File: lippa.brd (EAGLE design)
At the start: 50 x 80 mm, 149 parts, among them K1 629105136821, X1 B4B-PH-K-S, X10 PIIKKIRIMA-3, X11 B8B-PH-K-S, X2 B4B-PH-K-S, X3 B4B-PH-K-S, X4 B4B-PH-K-S, X5 LIITTIMET_X3815-10, X7 PIIKKIRIMA-3, X8 B6B-PH-K-S, X9 PIIKKIRIMA-3, Y1 EKE_PTH3.2-6.5SQ, Y2 EKE_PTH3.2-6.5SQ, Y3 EKE_PTH3.2-6.5SQ, Y4 EKE_PTH3.2-6.5SQ

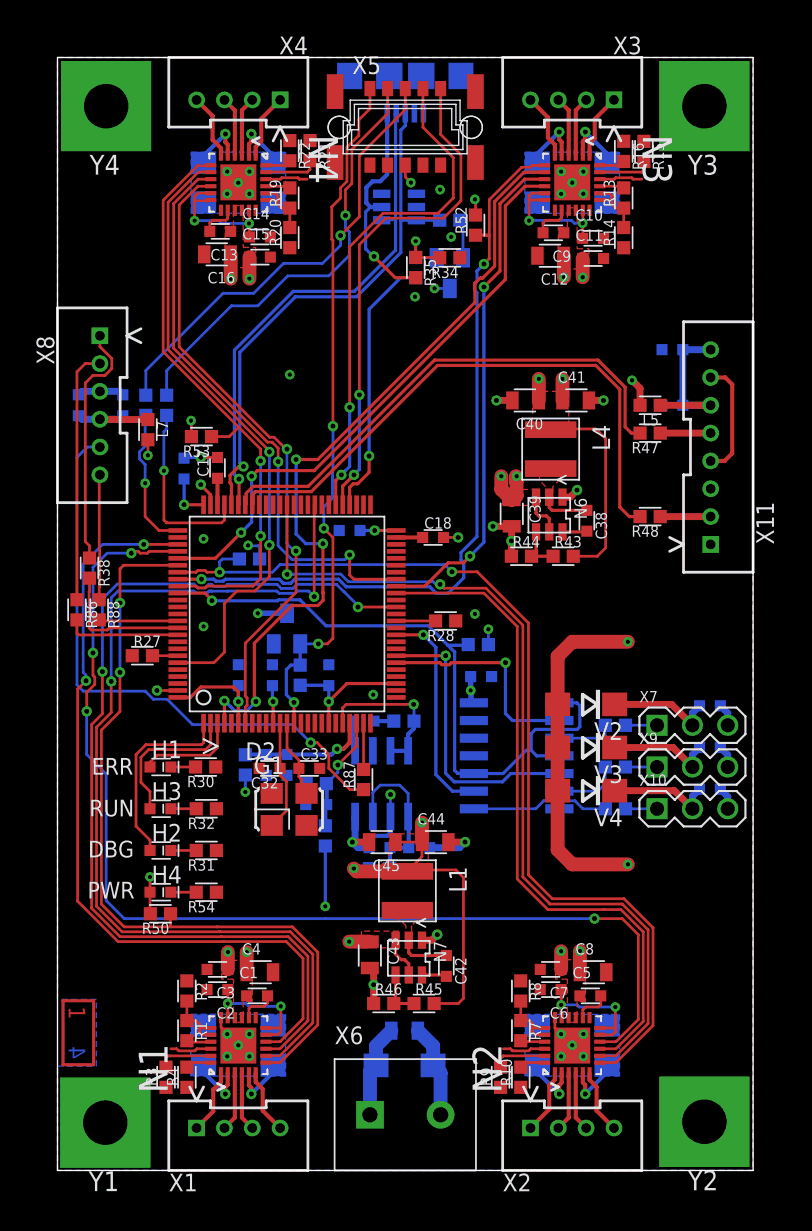
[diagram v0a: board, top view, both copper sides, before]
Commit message: Layout complete
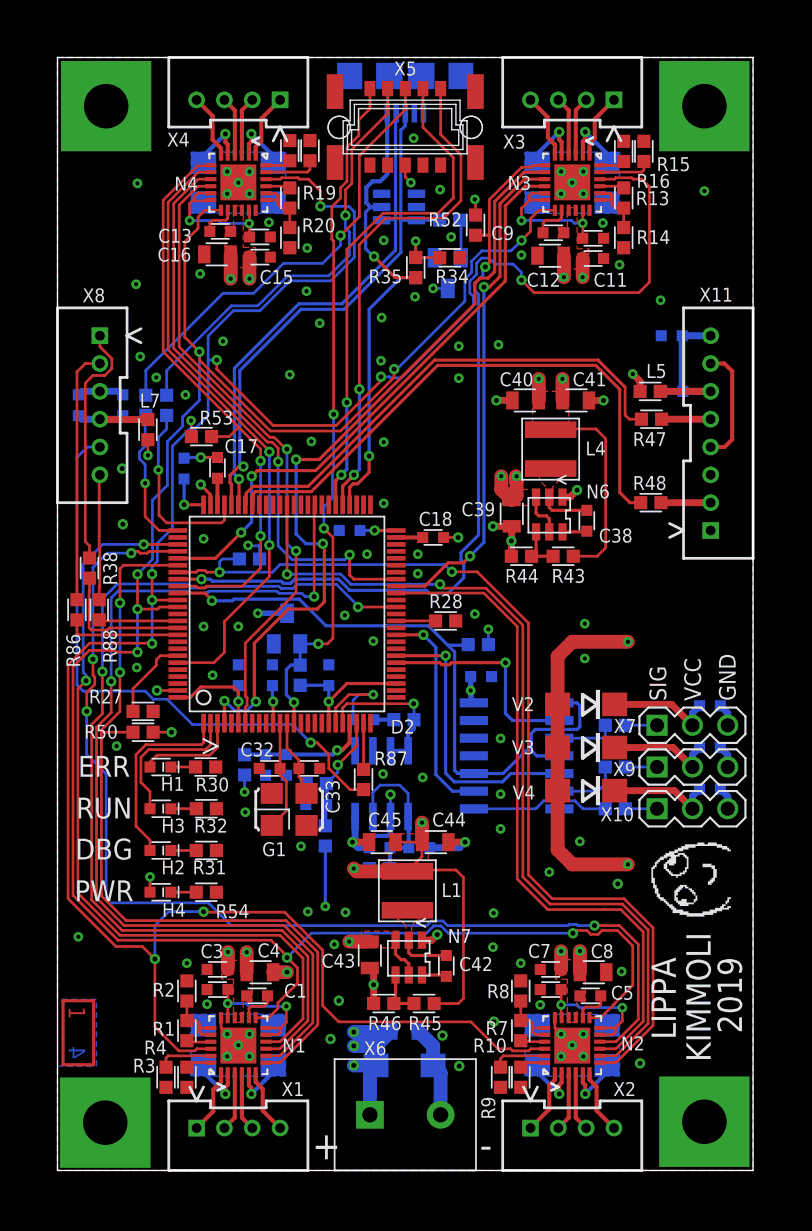
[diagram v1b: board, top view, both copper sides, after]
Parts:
- added U$1: DAFUG, lippa:DAFUG
- moved R50 13.1 mm to (6.15, 31.5), turned to 0 degrees
- moved R27 4.00 mm to (6.15, 33.0), turned to 180 degrees
- moved R47 1.00 mm to (42.7, 54.0)
- moved C48 1.00 mm to (44.1, 60.0)
- moved R48 1.00 mm to (42.6, 48.0)
- moved C46 1.00 mm to (44.2, 56.0)
- moved L5 1.00 mm to (42.6, 56.0)
- moved X11 1.00 mm to (47.5, 53.0)
- moved V1 0.15 mm to (28.1, 64.5)
- moved C21 0.10 mm to (22.0, 32.4)
- moved R26 0.10 mm to (24.9, 32.4)
- moved C19 0.05 mm to (16.4, 29.1)
- moved C20 0.05 mm to (14.9, 29.1)
- moved L2 0.05 mm to (13.4, 29.1)
- renumbered K1 to X12
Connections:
- net N$14 renamed SERVO_2
- net N$15 renamed SERVO_1
- net N$16 renamed SERVO_3
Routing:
- net SLEEP_N: track 12.2 -> 182.2 mm, vias 0 -> 9
- net FAULT_N: track 0.00 -> 154.9 mm, vias 0 -> 8
- net +VBAT: track 65.5 -> 73.8 mm, vias 14 -> 17
- net GND: track 53.5 -> 59.3 mm, vias 42 -> 109
- net BOOT0: track 1.83 -> 6.07 mm
- net USART1TX: track 41.9 -> 40.9 mm
- net ENA_1_N: track 56.9 -> 57.9 mm
- net USART1RX: track 37.0 -> 36.2 mm
- net VINT_3: track 10.1 -> 10.9 mm
- net USB_DP: track 39.2 -> 38.4 mm
- net USB_DM: track 36.7 -> 36.0 mm
- net PULSE_4: track 45.1 -> 44.3 mm
- net VINT_2: track 10.1 -> 10.8 mm
- net DIR_1: track 70.9 -> 70.3 mm
- net VINT_4: track 10.2 -> 10.7 mm
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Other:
- board text added: "+"
- board text added: "-"
- board text added: "2019"
- board text added: "KIMMOLI"
- board text added: "LIPPA"
- board text added: "SIG VCC GND"
